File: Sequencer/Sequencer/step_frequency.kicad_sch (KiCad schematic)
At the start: 4 parts

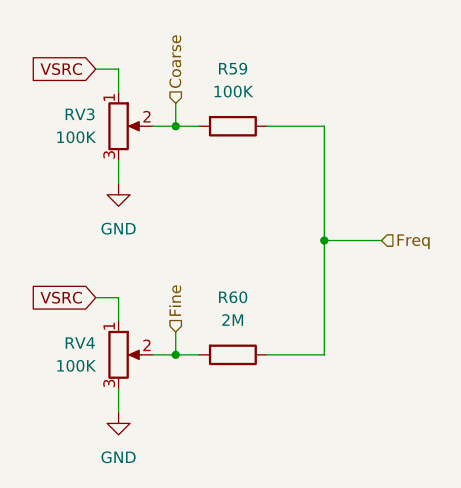
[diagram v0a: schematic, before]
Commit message: Sequencer - mostly positionned
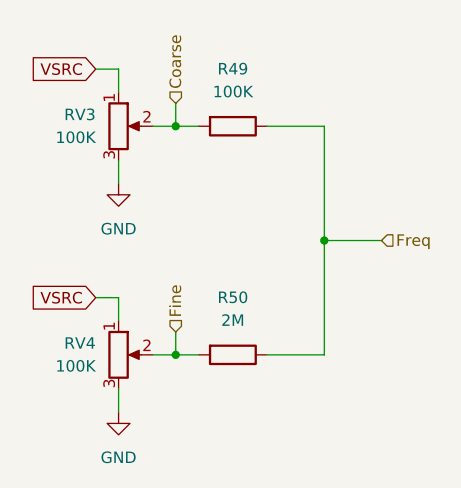
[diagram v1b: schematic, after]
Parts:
- renumbered R59 to R49, R60 to R50

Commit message: Sequencer - misc
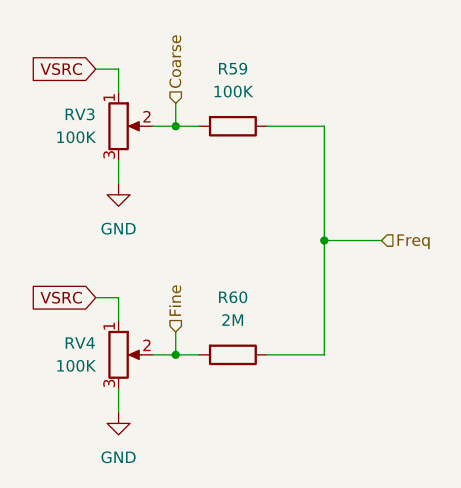
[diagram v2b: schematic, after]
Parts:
- renumbered R49 to R59, R50 to R60
